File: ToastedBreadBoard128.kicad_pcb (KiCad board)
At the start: 2 copper layers, 53.3 x 176.5 mm, 11 parts, among them J1 Conn_02x20_Odd_Even, J2 Conn_02x20_Odd_Even, J3 Conn_02x20_Odd_Even, J4 Conn_02x20_Odd_Even, J5 Conn_02x20_Odd_Even, J6 Conn_02x20_Odd_Even, U1 DIL126

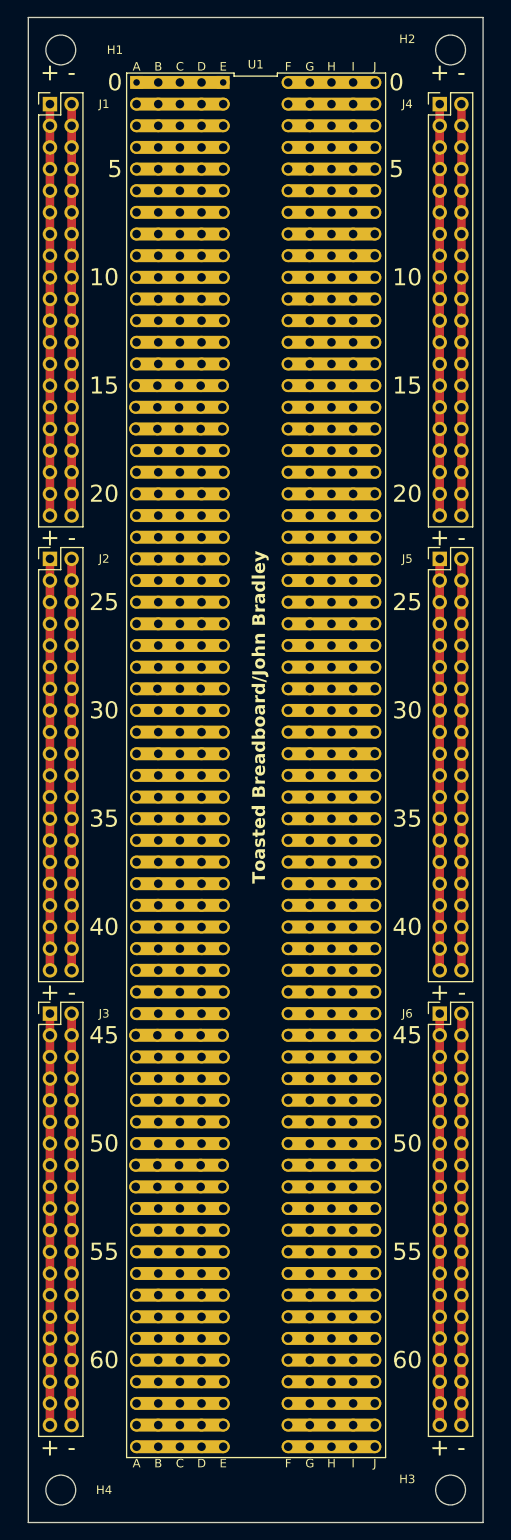
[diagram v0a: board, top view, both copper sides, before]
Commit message: Correct Width.
Signed-off-by: John Bradley <flypie@rocketmail.com>
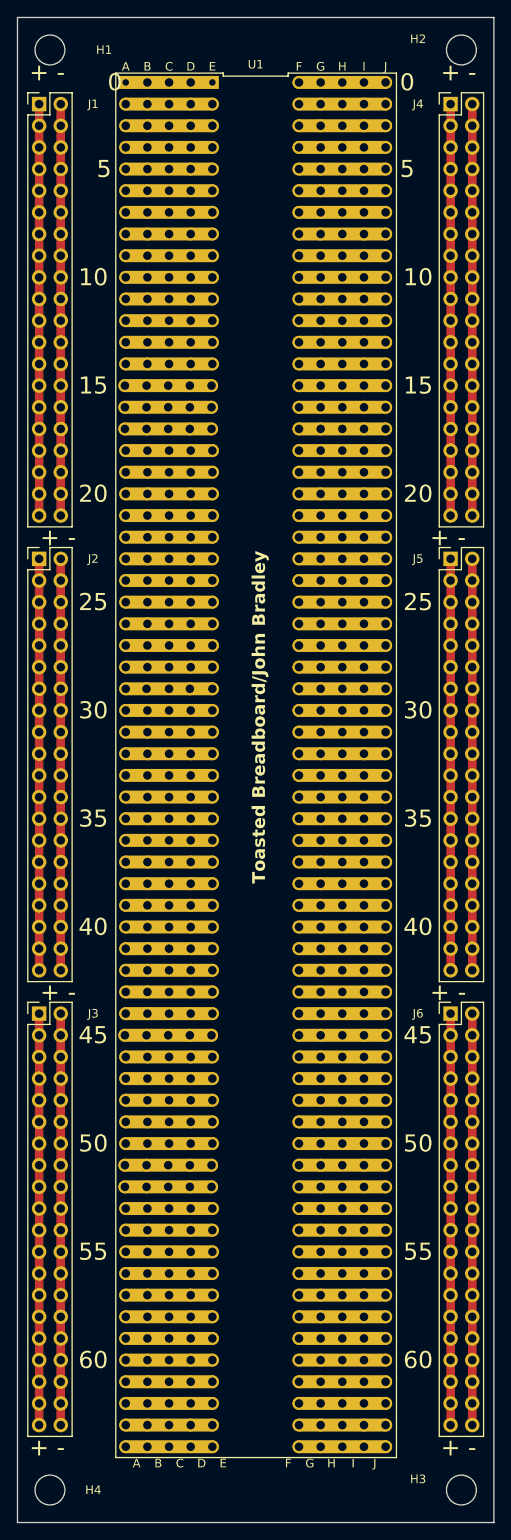
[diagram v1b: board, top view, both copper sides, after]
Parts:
- moved H2 1.27 mm to (152.4, 25.4)
- moved H3 1.27 mm to (152.4, 194.3)
- moved H1 1.27 mm to (104.1, 25.4)
- moved H4 1.27 mm to (104.1, 194.3)
- moved J1 1.27 mm to (102.9, 31.8)
- moved J2 1.27 mm to (102.9, 85.1)
- moved J3 1.27 mm to (102.9, 138.4)
- moved J4 1.27 mm to (151.1, 31.8)
- moved J5 1.27 mm to (151.1, 85.1)
- moved J6 1.27 mm to (151.1, 138.4)
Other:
- board size 53.3 x 176.5 mm -> 55.9 x 176.5 mm
